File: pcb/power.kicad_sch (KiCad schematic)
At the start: 33 parts, among them J1 Conn_01x03, Q1 AO3407A, SW1 POWER, U1 TPS2121RUXR, U2 TPS2121RUXR, U3 TPS2121RUXR, U4 74LVC1G08

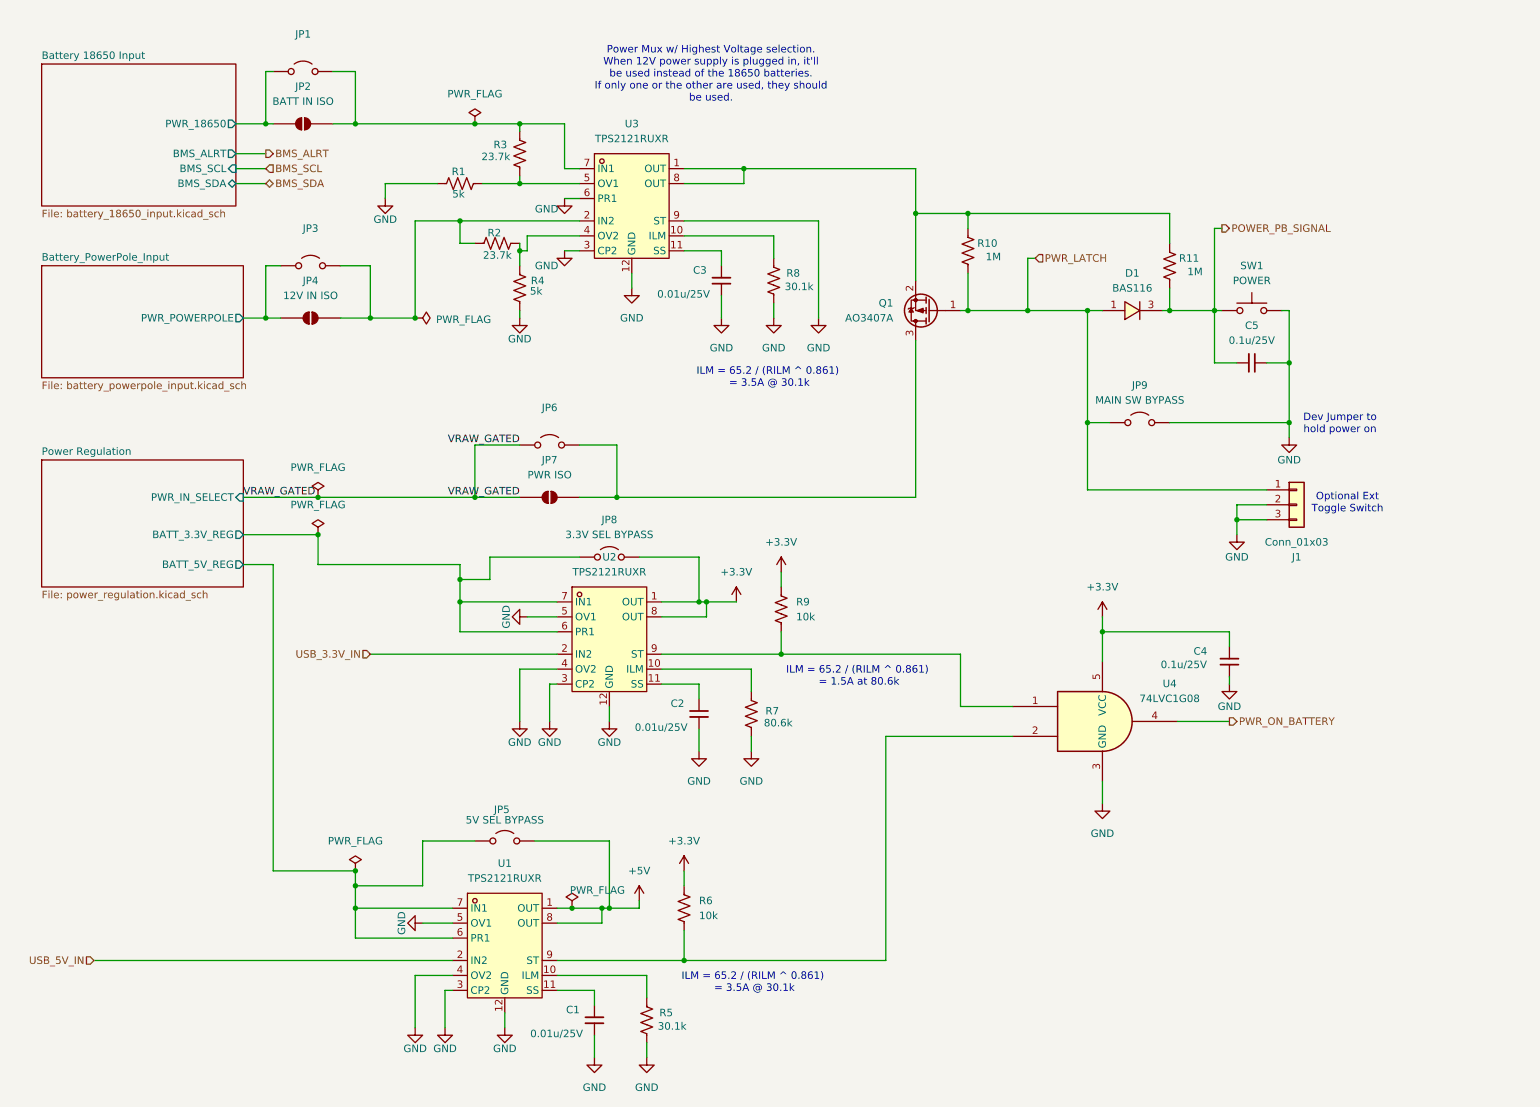
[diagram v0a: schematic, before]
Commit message: annotations
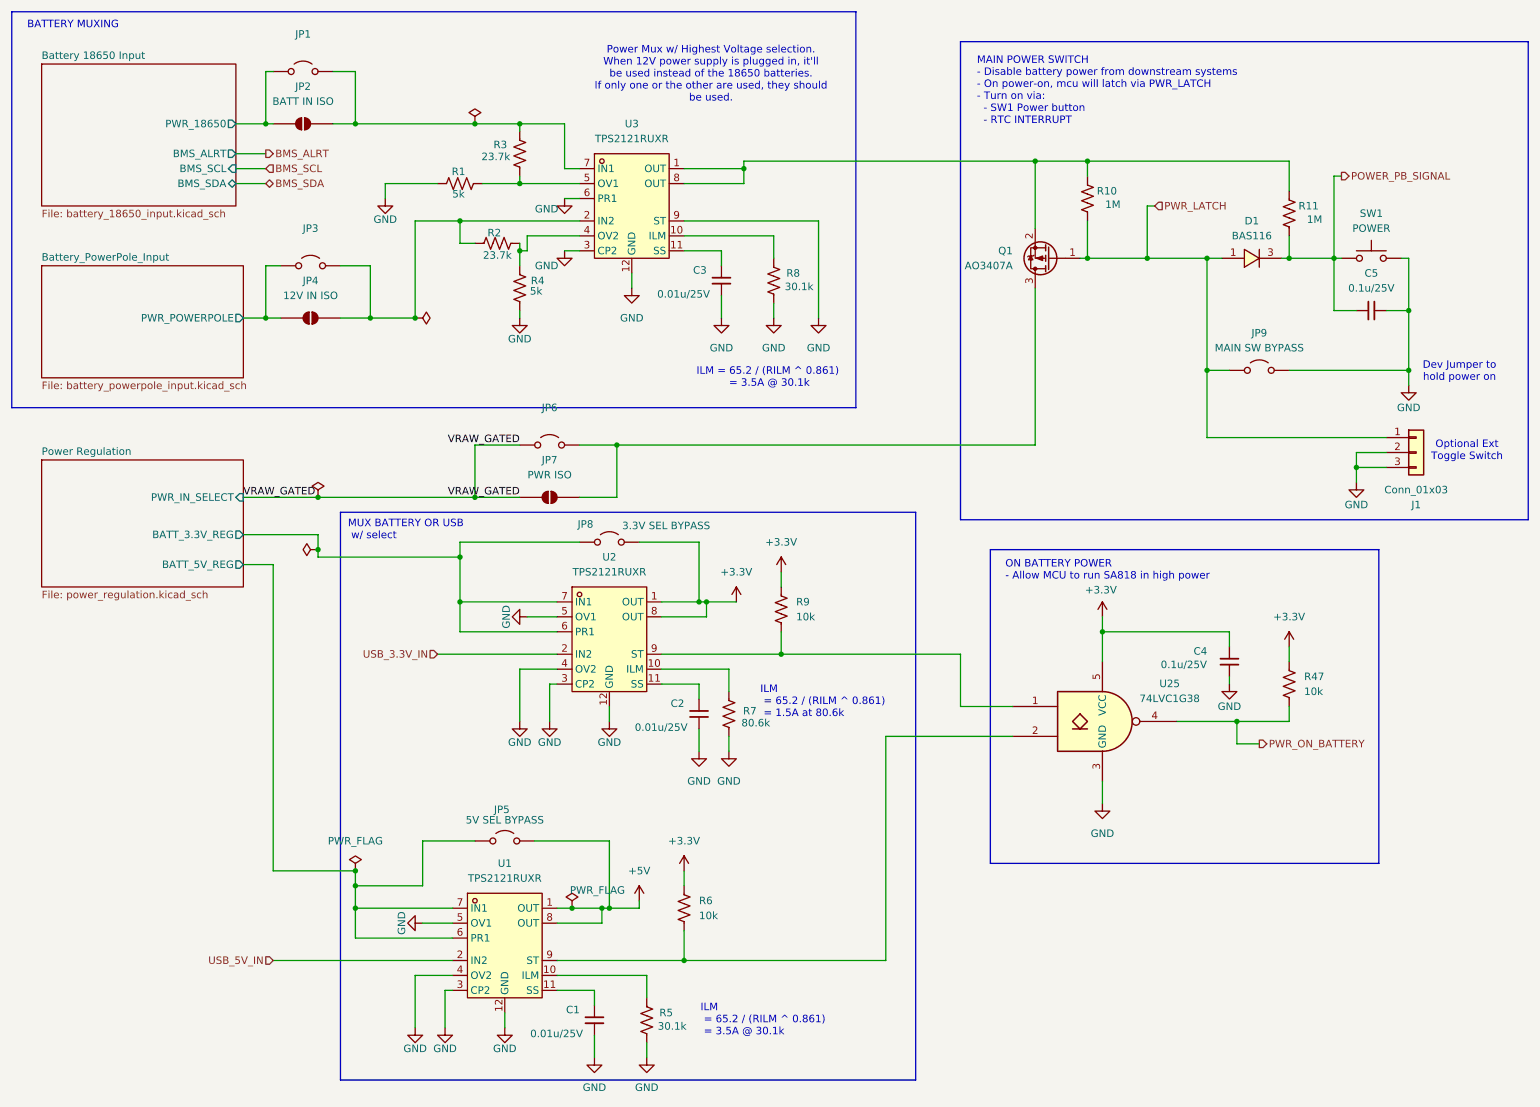
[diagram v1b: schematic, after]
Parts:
- removed U4: 74LVC1G08, Package_TO_SOT_SMD:SOT-23-5, symbol 74xGxx:74LVC1G08
- added R47: 10k, Resistor_SMD:R_0603_1608Metric, symbol Device:R_US
- added U25: 74LVC1G38, Package_TO_SOT_SMD:SOT-23-5, symbol 74xGxx:74LVC1G38
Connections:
- net +3.3V: now also R47.2, U25.5 (VCC)
- net GND: now also U25.3 (GND)
- net PWR_ON_BATTERY: now also R47.1, U25.4
- net at R9.1, U2.9 (ST): now also U25.1
- net at R6.1, U1.9 (ST): now also U25.2
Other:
- note added: "BATTERY MUXING"
- note added: "MAIN POWER SWITCH - Disable battery power from downstream systems - On power-on, mcu will latch via PWR_LATCH - Turn on via: - SW1 Power button - RTC INTERRUPT"
- note added: "MUX BATTERY OR USB w/ select"
- note added: "ON BATTERY POWER - Allow MCU to run SA818 in high power"
- moved on the sheet: C5, D1, J1, JP8, JP9, Q1, R10, R11, R7, SW1
